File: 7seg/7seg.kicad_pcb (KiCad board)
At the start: 2 copper layers, 110.5 x 43.2 mm, 26 parts, among them IC1 ATTINY88-AZ, P1 TST, P2 TST, P3 SPI, P4 TST, P5 TST, Q1 MBT3904DW1, Q10 MBT3904DW1, Q2 MBT3904DW1, Q3 MBT3904DW1, Q4 MBT3904DW1, Q5 MBT3904DW1, Q6 MBT3904DW1, Q7 MBT3904DW1, Q8 MBT3904DW1, Q9 MBT3904DW1, U1 TLC6C5912

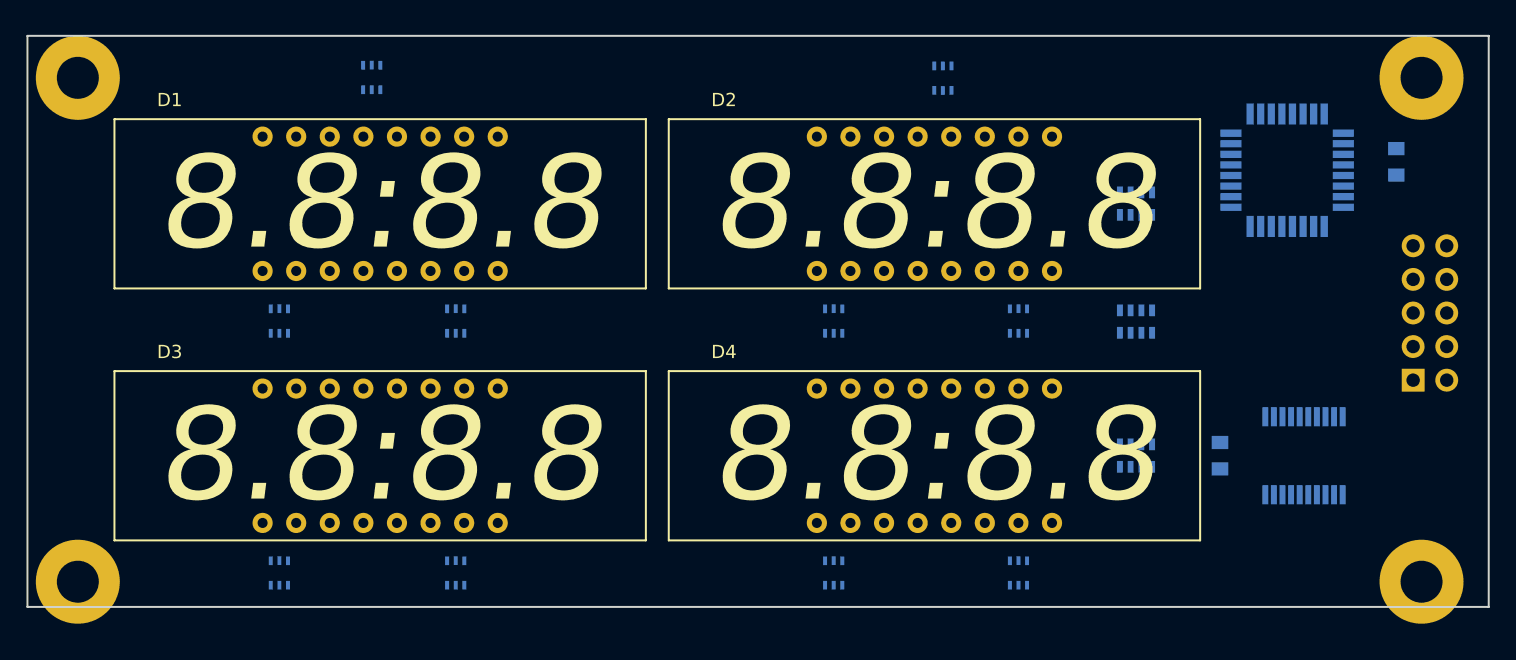
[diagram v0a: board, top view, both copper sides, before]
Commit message: spin 7seg board and io 2.5
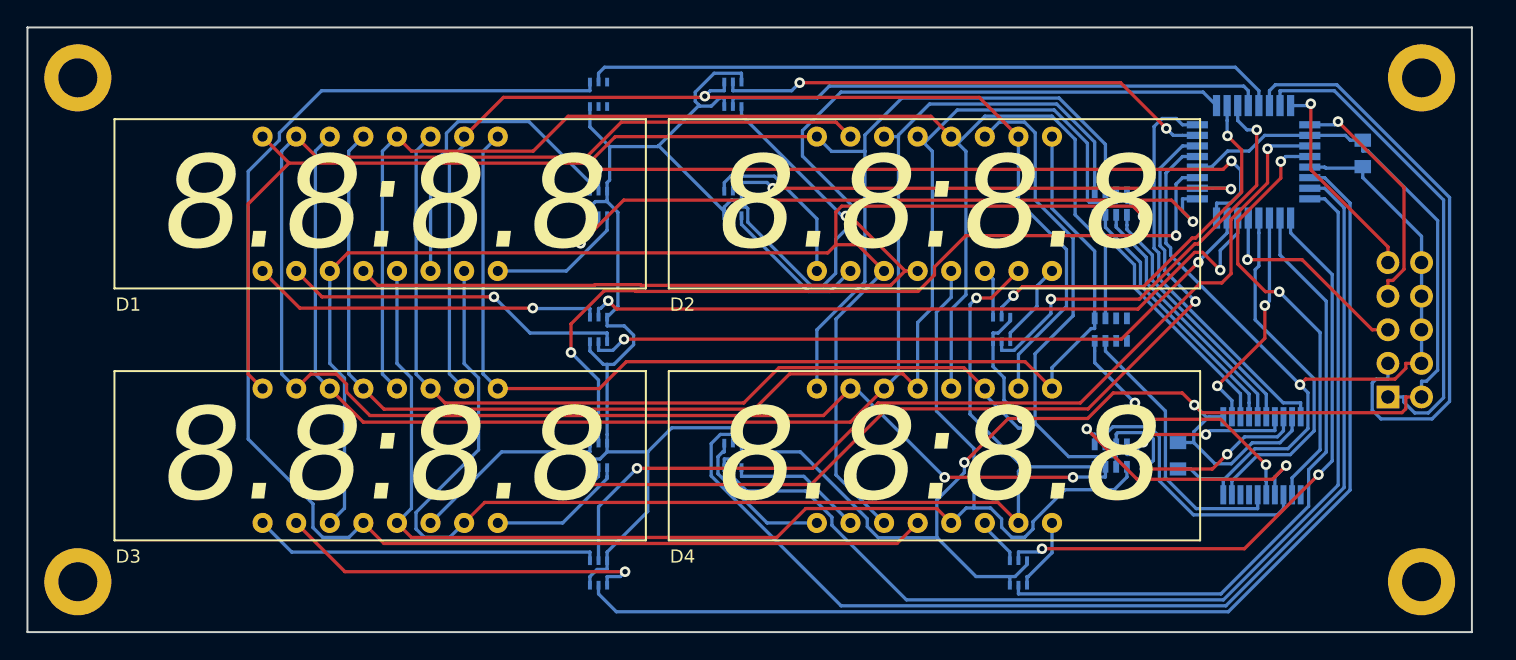
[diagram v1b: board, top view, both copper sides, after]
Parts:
- moved Q1 24.1 mm to (124.5, 97.2)
- moved Q6 24.1 mm to (124.5, 115.6)
- moved Q10 17.2 mm to (124.5, 79.4)
- moved Q5 15.9 mm to (134.6, 79.4), turned to 0 degrees
- moved Q2 14.0 mm to (124.5, 87.6)
- moved Q7 14.0 mm to (124.5, 106.7)
- moved Q3 11.7 mm to (134.6, 87.6)
- moved Q8 11.7 mm to (134.6, 106.7)
- moved U1 3.18 mm to (174.6, 106.7)
- moved C3 3.17 mm to (168.3, 106.7)
- moved C2 2.62 mm to (182.2, 83.8)
- moved IC1 2.62 mm to (174.0, 84.5)
- moved P3 2.29 mm to (184.2, 102.2)
- moved RP1 2.01 mm to (163.2, 97.2), turned to 0 degrees
- moved RP2 1.91 mm to (163.2, 106.7)
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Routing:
- net +5V: track 0.00 -> 224.6 mm, vias 0 -> 3
- net Net-(D1-Pad15): track 0.00 -> 131.8 mm, vias 0 -> 2
- net Net-(D1-Pad3): track 0.00 -> 114.2 mm, vias 0 -> 1
- net Net-(D1-Pad16): track 0.00 -> 111.5 mm
- net Net-(D1-Pad12): track 0.00 -> 109.0 mm
- net Net-(D1-Pad11): track 0.00 -> 106.4 mm
- net Net-(D3-Pad4): track 0.00 -> 106.1 mm
- net Net-(D1-Pad13): track 0.00 -> 105.8 mm
- net Net-(D1-Pad14): track 0.00 -> 105.5 mm
- net Net-(D1-Pad5): track 0.00 -> 101.3 mm
- net Net-(D1-Pad7): track 0.00 -> 97.9 mm, vias 0 -> 1
- net Net-(D1-Pad10): track 0.00 -> 88.8 mm, vias 0 -> 1
- net /Digit9: track 0.00 -> 87.4 mm
- net Net-(D1-Pad9): track 0.00 -> 85.4 mm
- net /Digit12: track 0.00 -> 85.0 mm
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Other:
- board size 110.5 x 43.2 mm -> 109.2 x 45.7 mm
